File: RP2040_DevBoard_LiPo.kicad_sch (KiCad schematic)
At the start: 55 parts, among them J1 HRO_TYPE-C-31-M-14, J3 Conn_01x18, J4 Conn_01x18, Q1 DMP2045U, SW1 SW_Push, SW2 SW_Push, U1 W25Q128JVS, U2 SRV05-4, U3 RP2040, U5 SOT23-5 200mA 3.3V, Y1 Crystal_GND23

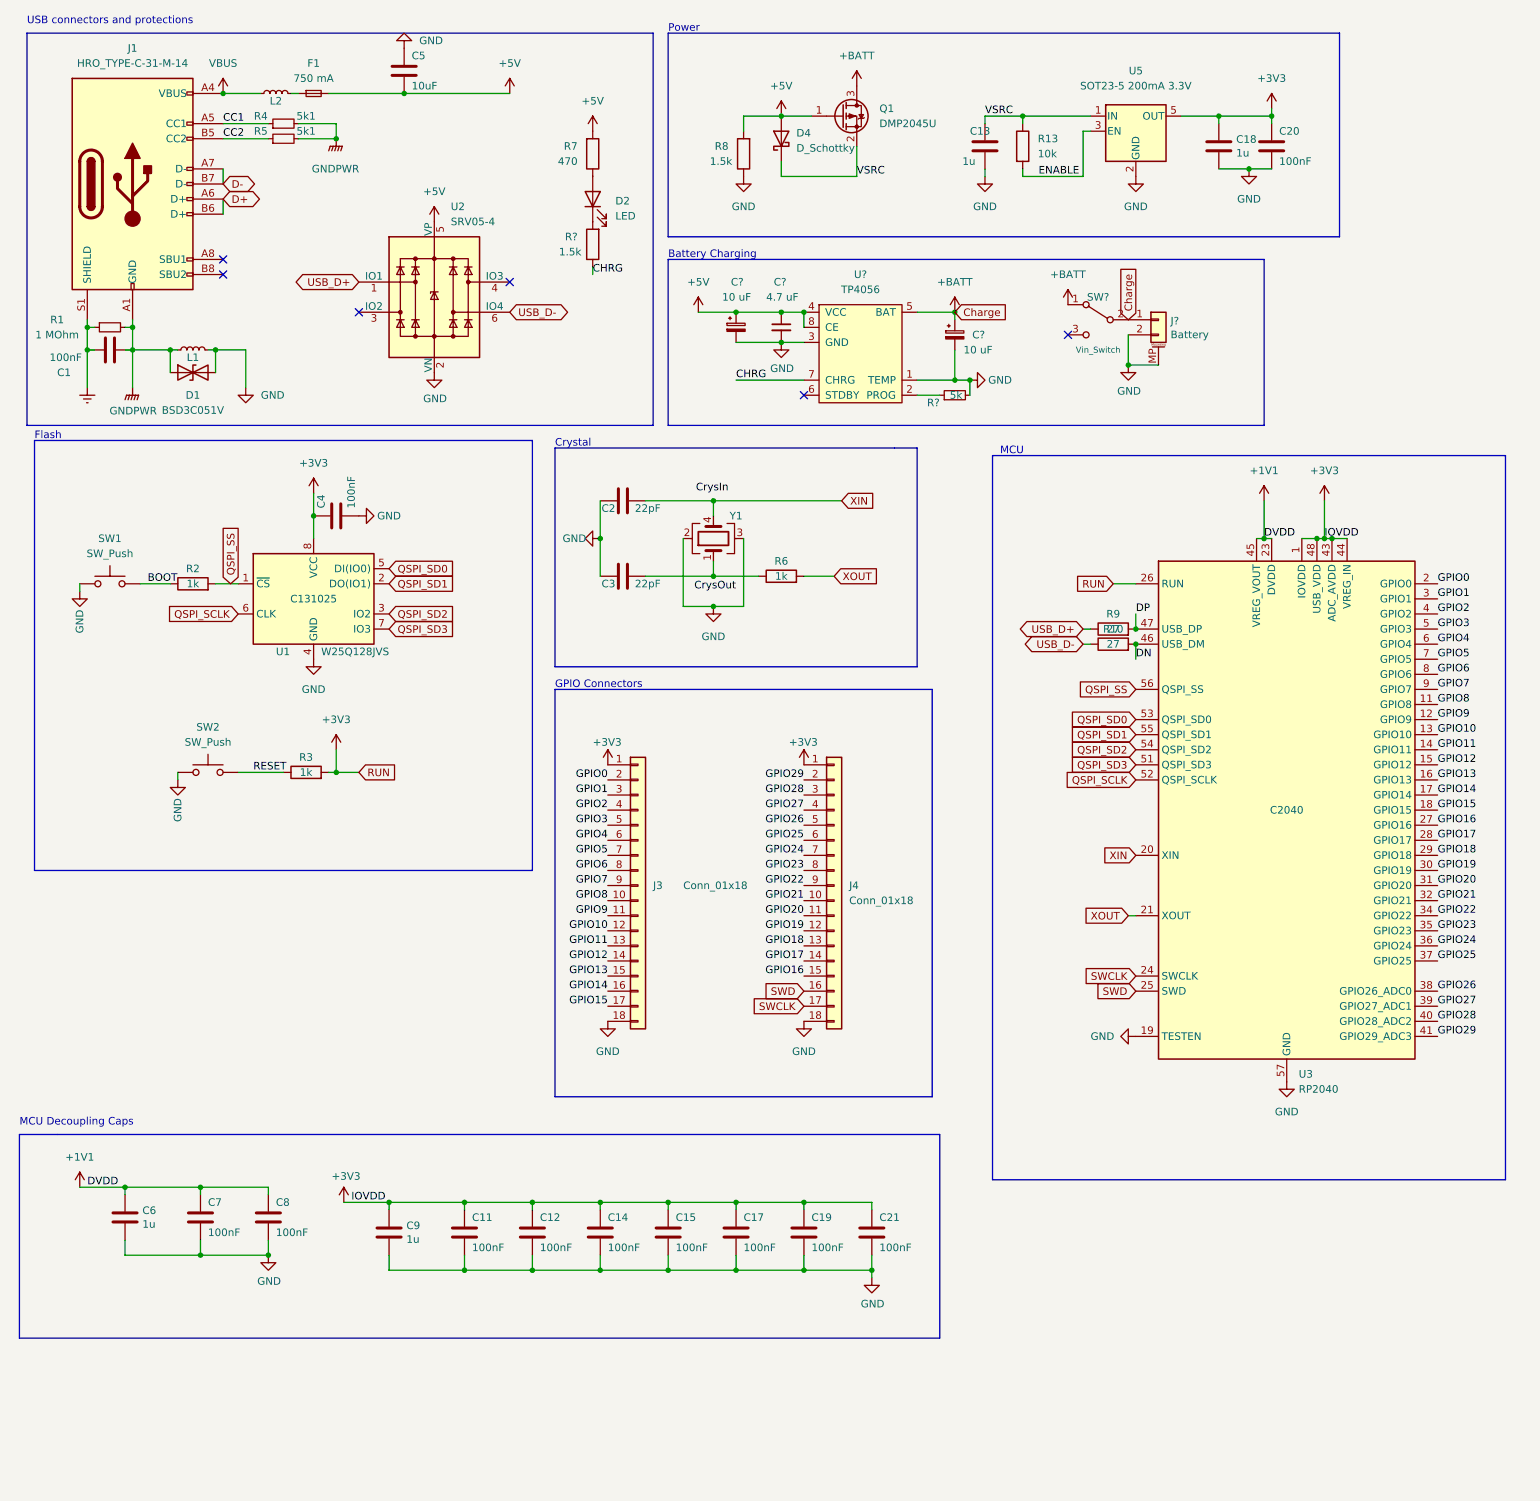
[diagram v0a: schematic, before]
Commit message: started routing
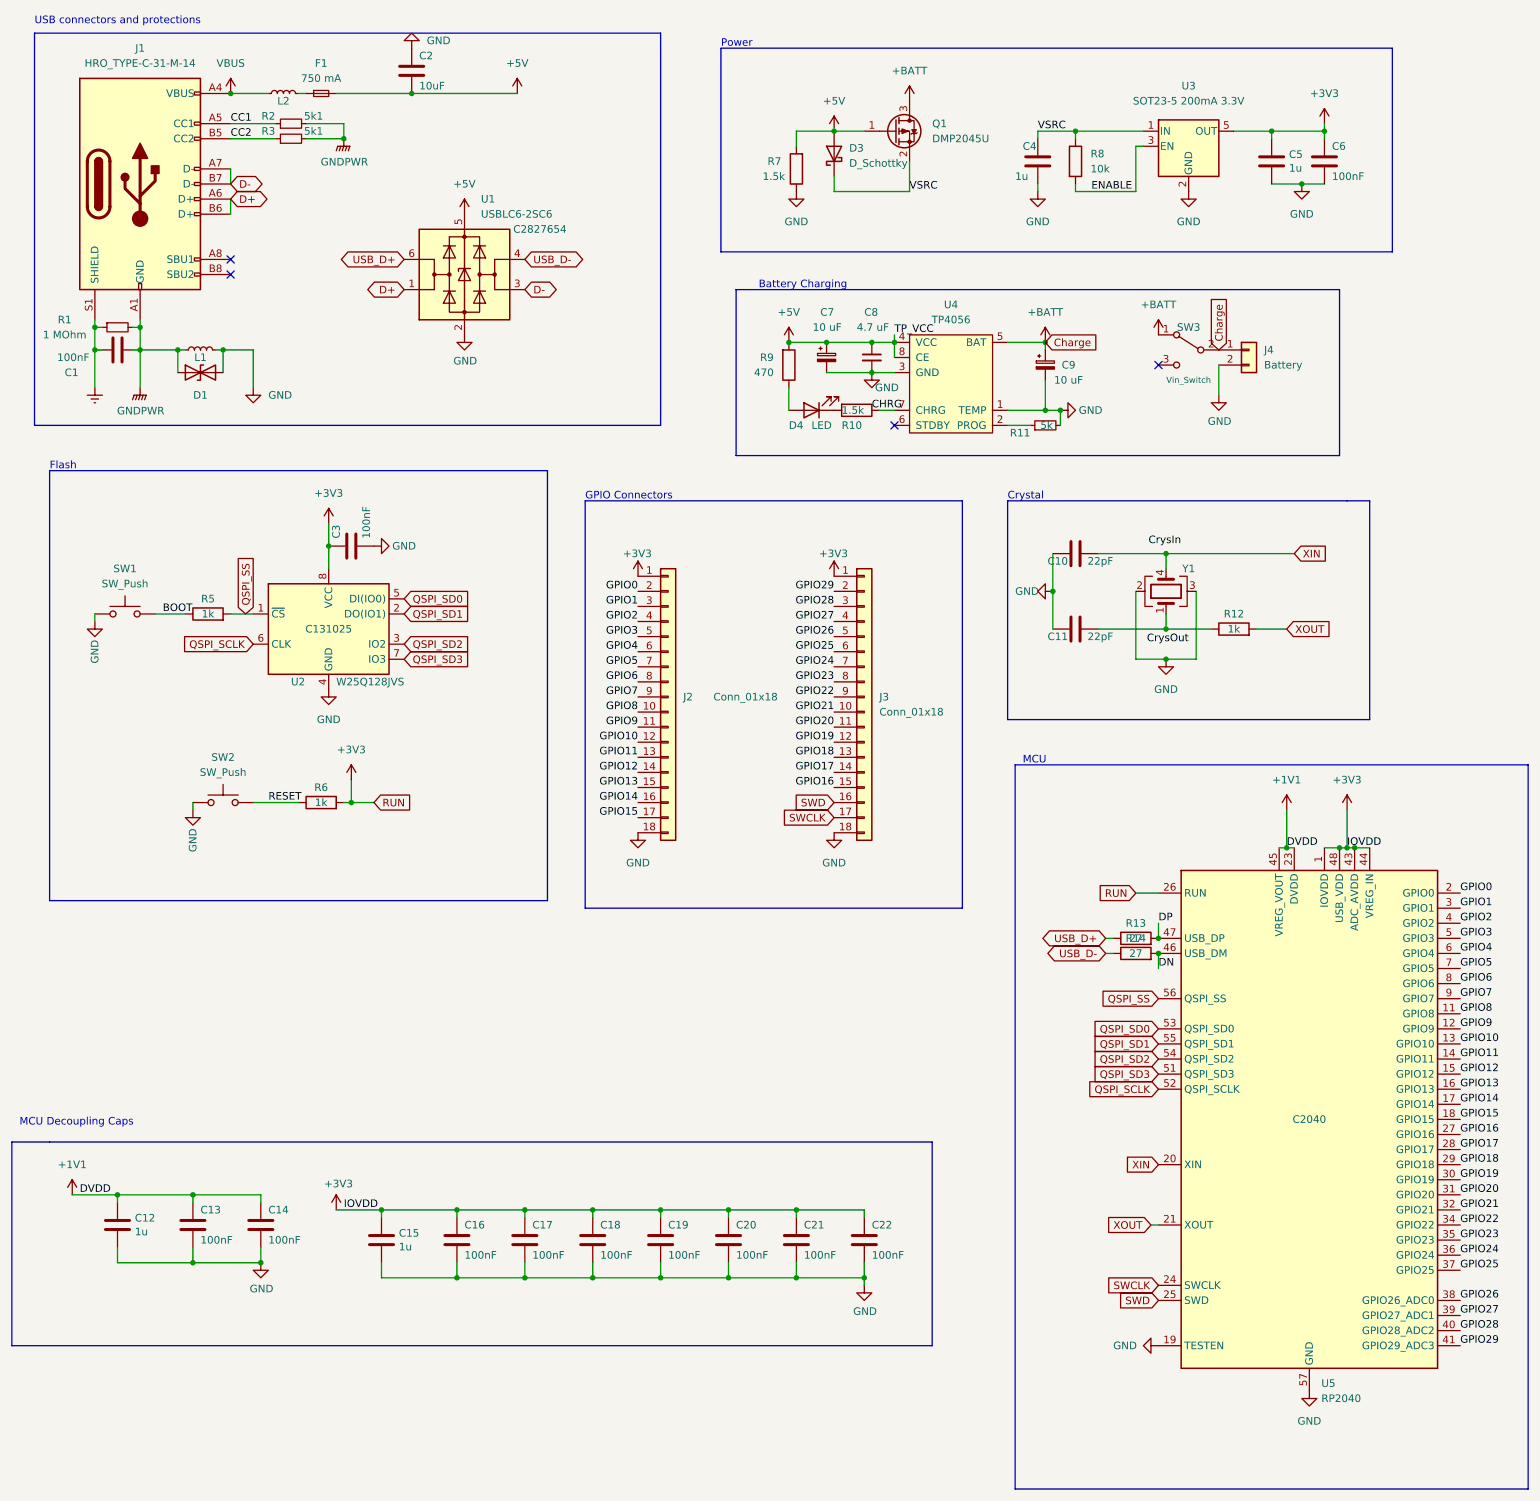
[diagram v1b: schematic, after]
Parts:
- removed D2: LED, LED_SMD:LED_1206_3216Metric, symbol Device:LED
- removed J?: Battery, Connector_JST:JST_PH_S2B-PH-K_1x02_P2.00mm_Horizontal, symbol Connector_Generic_MountingPin:Conn_01x02_MountingPin
- removed R7: 470, Resistor_SMD:R_0402_1005Metric, symbol Device:R
- removed U2: SRV05-4, Package_TO_SOT_SMD:SOT-23-6, symbol Power_Protection:SRV05-4
- added D4: LED, LED_SMD:LED_1206_3216Metric, symbol Device:LED
- added J4: Battery, Connector_JST:JST_EH_S2B-EH_1x02_P2.50mm_Horizontal, symbol Connector_Generic:Conn_01x02
- added R9: 470, Resistor_SMD:R_0402_1005Metric, symbol Device:R
- added U1: USBLC6-2SC6, Package_TO_SOT_SMD:SOT-23-6, symbol Power_Protection:USBLC6-2SC6
- gave numbers to parts that had none: 7
- renumbered C2 to C10, C3 to C11, C6 to C12, C7 to C13, C8 to C14, C9 to C15, C11 to C16, C12 to C17, C14 to C18, C15 to C19, C5 to C2, C17 to C20, C19 to C21, C21 to C22, C4 to C3, C13 to C4, C18 to C5, C20 to C6, D4 to D3, J3 to J2, J4 to J3, R6 to R12, R9 to R13, R10 to R14, R4 to R2, R5 to R3, R2 to R5, R3 to R6, R8 to R7, R13 to R8, U1 to U2, U5 to U3, U3 to U5
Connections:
- net +5V: now also R9.2, U1.5 (VBUS)
- net +BATT: now also J4.1 (Pin_1)
- net CHRG: no longer R10.1, U4.7 (CHRG)
- net D+: now also U1.1 (I/O1)
- net D-: now also U1.3 (I/O2)
- net GND: now also J4.2 (Pin_2), U1.2 (GND)
- net USB_D+: now also U1.6 (I/O1)
- net USB_D-: now also U1.4 (I/O2)
- net at R10.2: now also D4.1 (K)
- new net: R10.1, U4.7 (CHRG)
- new net: D4.2 (A), R9.1
- no-connect marks 6 -> 4
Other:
- moved on the sheet: C1, C10, C11, C12, C13, C14, C15, C16, C17, C18, C19, C2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
